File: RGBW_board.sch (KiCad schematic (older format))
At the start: 13 parts, among them J1 Jack-DC, J2 Conn_01x02, J3 Conn_01x04, J4 Conn_01x02, Q1 2N7002, Q2 2N7002, Q3 2N7002, Q4 2N7002, U1 WeMos_mini

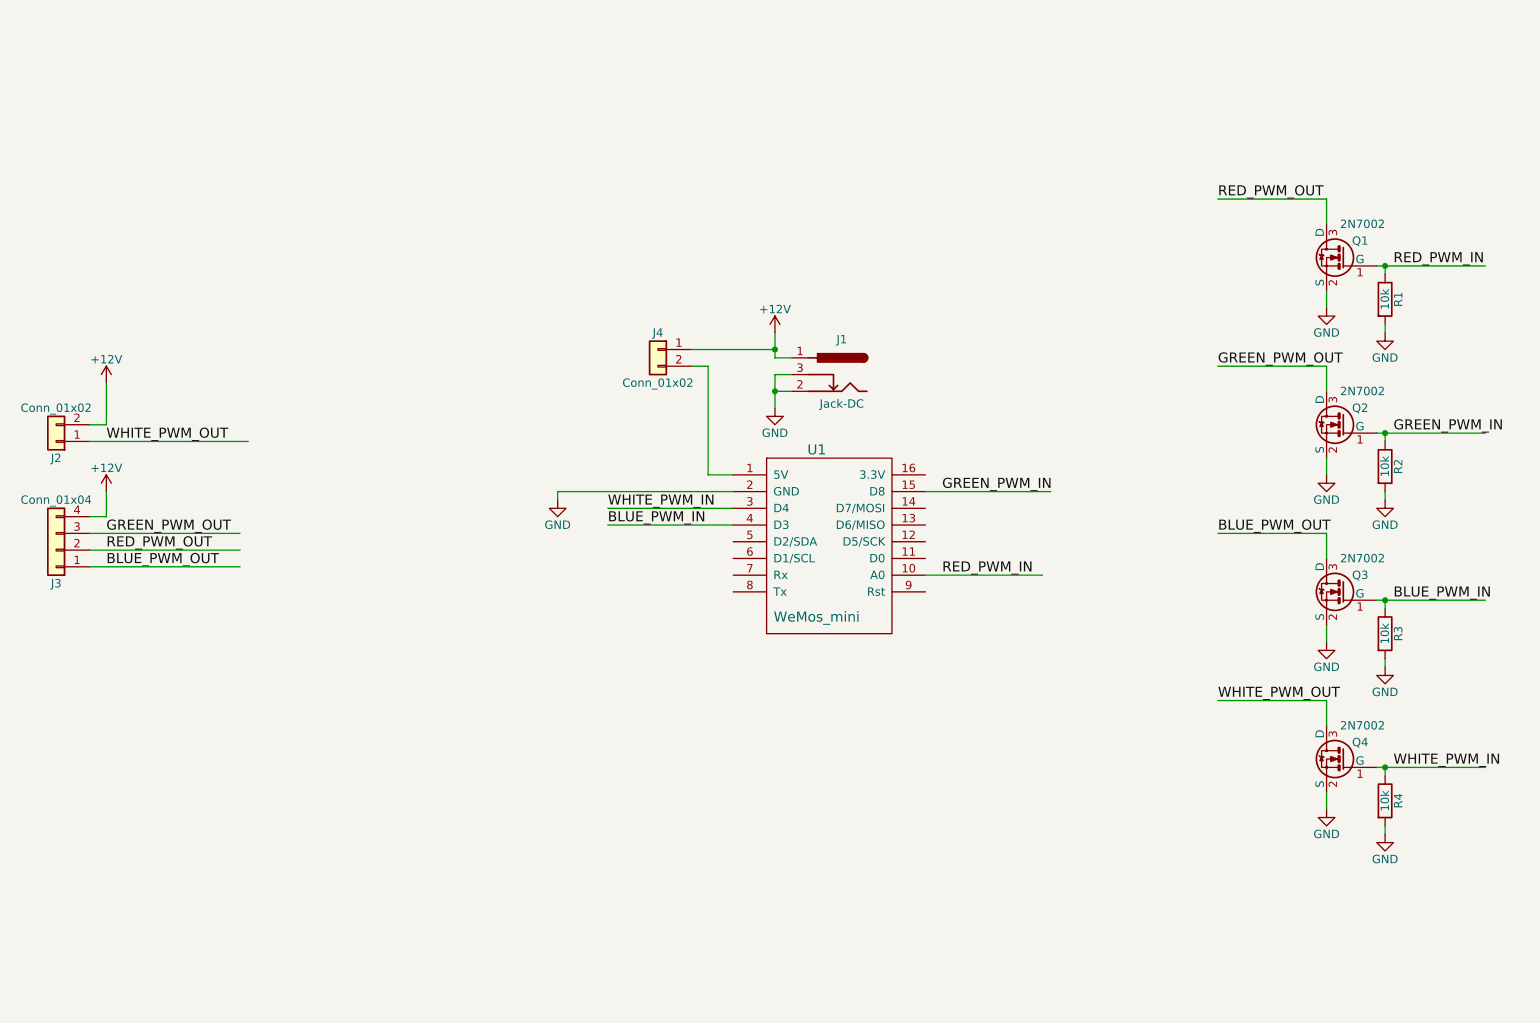
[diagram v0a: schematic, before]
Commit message: --REV1-- Added rev1 to project git
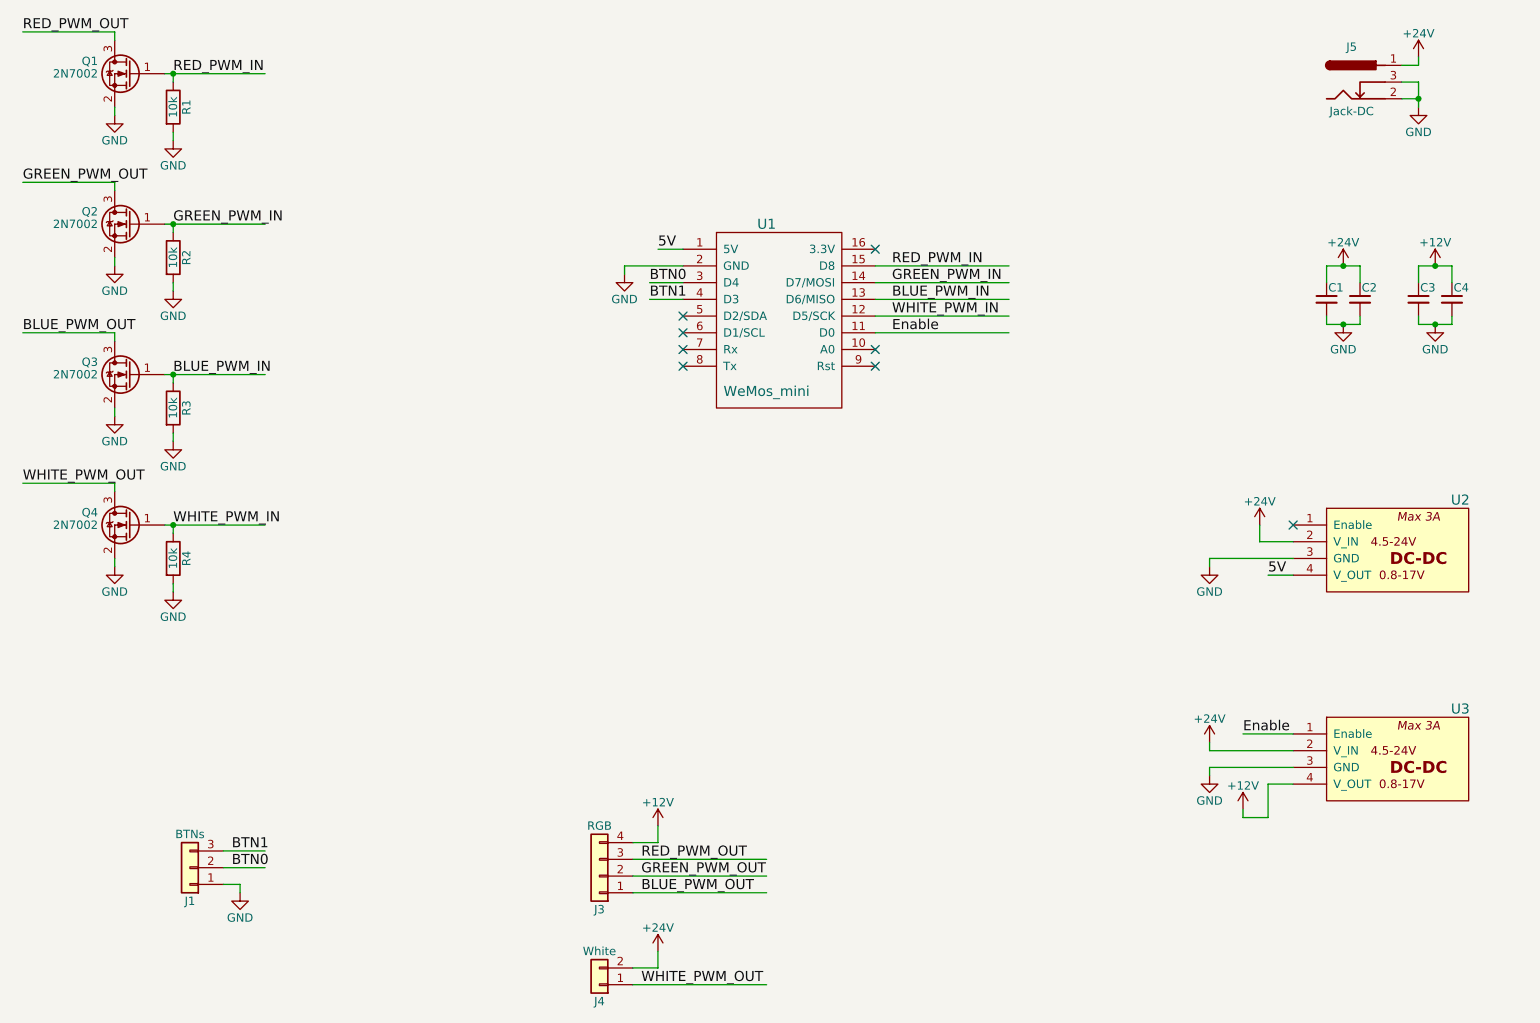
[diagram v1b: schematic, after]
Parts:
- removed J1: Jack-DC, Connectors:BARREL_JACK, symbol Jack-DC
- removed J2: Conn_01x02, Pin_Headers:Pin_Header_Angled_1x02_Pitch2.54mm, symbol Conn_01x02
- removed Q1, Q2, Q3, Q4: 2N7002, TO_SOT_Packages_SMD:SOT-23, symbol 2N7002-RESCUE-RGBW_board
- added C1, C2, C3, C4: C_Small, Capacitors_SMD:C_1210, symbol C_Small
- added J1: BTNs, Connectors_Molex:Molex_KK-6410-03_03x2.54mm_Straight, symbol Conn_01x03
- added J5: Jack-DC, Connectors:BARREL_JACK, symbol Jack-DC
- added Q1, Q2, Q3, Q4: 2N7002, TO_SOT_Packages_SMD:SOT-23, symbol 2N7002
- added U2, U3: Mini_DC-DC_4.5-24V_to_0.8-17V, kenneth:Mini_DC-DC_converter, symbol Mini_DC-DC_4.5-24V_to_0.8-17V
- J3: value Conn_01x04 -> RGB; footprint Pin_Headers:Pin_Header_Angled_1x04_Pitch2.54mm -> Connectors_Molex:Molex_KK-6410-04_04x2.54mm_Straight
- J4: value Conn_01x02 -> White; footprint Pin_Headers:Pin_Header_Angled_1x02_Pitch2.54mm -> Connectors_Molex:Molex_KK-6410-02_02x2.54mm_Straight
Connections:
- net labels added: +24V, 5V, BTN0, BTN1, Enable
- wire segments 47 -> 77
- no-connect marks 0 -> 8
